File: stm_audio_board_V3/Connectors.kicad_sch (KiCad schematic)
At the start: 6 parts, among them J2 STlink_DISP_MCU, J2 STlink_DSP

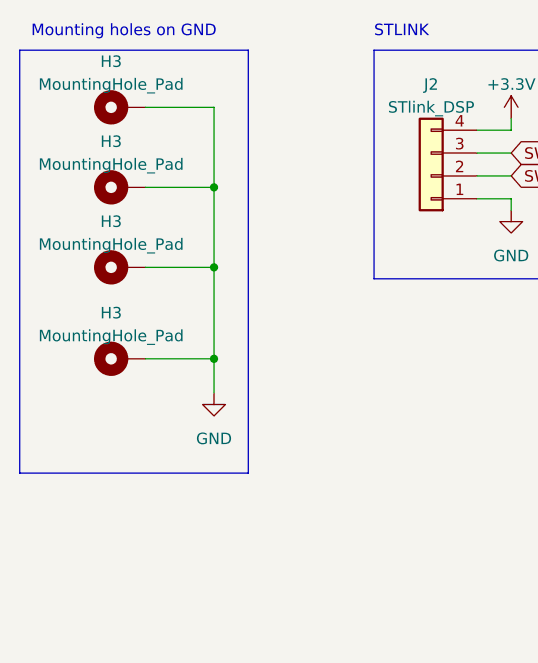
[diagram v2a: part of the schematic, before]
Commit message: PCB design is finished
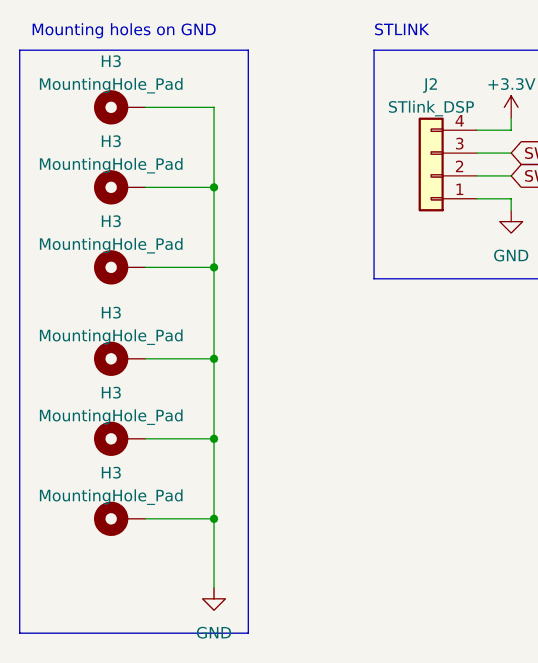
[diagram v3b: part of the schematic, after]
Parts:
- added H3 (x2): MountingHole_Pad, MountingHole:MountingHole_3.2mm_M3_DIN965_Pad, symbol Mechanical:MountingHole_Pad
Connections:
- net GND: now also H3.1, H3.1
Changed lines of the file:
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@@
   (junction (at 113.03 48.26) (diameter 0) (color 0 0 0 0)
   )
+  (junction (at 113.03 76.2) (diameter 0) (color 0 0 0 0)
+  )
+  (junction (at 113.03 67.31) (diameter 0) (color 0 0 0 0)
+  )
   (junction (at 113.03 39.37) (diameter 0) (color 0 0 0 0)
   )
-  (wire (pts (xy 113.03 62.23) (xy 113.03 58.42))
+  (wire (pts (xy 113.03 83.82) (xy 113.03 76.2))
     (stroke (width 0) (type default))
   )
@@
     (stroke (width 0) (type default))
   )
+  (wire (pts (xy 105.41 76.2) (xy 113.03 76.2))
+    (stroke (width 0) (type default))
+  )
+  (wire (pts (xy 113.03 76.2) (xy 113.03 67.31))
+    (stroke (width 0) (type default))
+  )
+  (wire (pts (xy 105.41 67.31) (xy 113.03 67.31))
+    (stroke (width 0) (type default))
+  )
   (wire (pts (xy 105.41 48.26) (xy 113.03 48.26))
     (stroke (width 0) (type default))
@@
     (stroke (width 0) (type default))
   )
+  (wire (pts (xy 113.03 67.31) (xy 113.03 58.42))
+    (stroke (width 0) (type default))
+  )
   (wire (pts (xy 142.24 33.02) (xy 146.05 33.02))
     (stroke (width 0) (type default))
@@
   )
   (text_box ""
-    (at 91.44 24.13 0) (size 25.4 46.99)
+    (at 91.44 24.13 0) (size 25.4 64.77)
     (stroke (width 0) (type default))
     (fill (type none))
@@
     )
   )
+  (symbol (lib_id "Mechanical:MountingHole_Pad") (at 102.87 67.31 90) (unit 1)
+    (in_bom yes) (on_board yes) (dnp no) (fields_autoplaced)
+    (property "Reference" "H3" (at 101.6 62.23 90)
+      (effects (font (size 1.27 1.27)))
+    )
+    (property "Value" "MountingHole_Pad" (at 101.6 64.77 90)
+      (effects (font (size 1.27 1.27)))
+    )
+    (property "Footprint" "MountingHole:MountingHole_3.2mm_M3_DIN965_Pad" (at 102.87 67.31 0)
+      (effects (font (size 1.27 1.27)) hide)
+    )
+    (property "Datasheet" "~" (at 102.87 67.31 0)
+      (effects (font (size 1.27 1.27)) hide)
+    )
+    (pin "1")
+    (instances
+      (project "stm_audio_board_V3"
+        (path "/6997cf63-2615-4e49-9471-e7da1b6bae71"
+          (reference "H3") (unit 1)
+        )
+        (path "/6997cf63-2615-4e49-9471-e7da1b6bae71/2eb2ee8f-ab98-4666-97f0-bfacb073bc88"
+          (reference "H4") (unit 1)
+        )
+        (path "/6997cf63-2615-4e49-9471-e7da1b6bae71/6424856c-1346-4018-a943-0d16008c9545"
+          (reference "H5") (unit 1)
+        )
+      )
+    )
+  )
   (symbol (lib_id "Mechanical:MountingHole_Pad") (at 102.87 58.42 90) (unit 1)
     (in_bom yes) (on_board yes) (dnp no) (fields_autoplaced)
@@
         (path "/6997cf63-2615-4e49-9471-e7da1b6bae71/6424856c-1346-4018-a943-0d16008c9545"
           (reference "#PWR034") (unit 1)
+        )
+      )
+    )
+  )
+  (symbol (lib_id "Mechanical:MountingHole_Pad") (at 102.87 76.2 90) (unit 1)
+    (in_bom yes) (on_board yes) (dnp no) (fields_autoplaced)
+    (property "Reference" "H3" (at 101.6 71.12 90)
+      (effects (font (size 1.27 1.27)))
+    )
+    (property "Value" "MountingHole_Pad" (at 101.6 73.66 90)
+      (effects (font (size 1.27 1.27)))
+    )
+    (property "Footprint" "MountingHole:MountingHole_3.2mm_M3_DIN965_Pad" (at 102.87 76.2 0)
+      (effects (font (size 1.27 1.27)) hide)
+    )
+    (property "Datasheet" "~" (at 102.87 76.2 0)
+      (effects (font (size 1.27 1.27)) hide)
+    )
+    (pin "1")
+    (instances
+      (project "stm_audio_board_V3"
+        (path "/6997cf63-2615-4e49-9471-e7da1b6bae71"
+          (reference "H3") (unit 1)
+        )
+        (path "/6997cf63-2615-4e49-9471-e7da1b6bae71/2eb2ee8f-ab98-4666-97f0-bfacb073bc88"
+          (reference "H4") (unit 1)
+        )
+        (path "/6997cf63-2615-4e49-9471-e7da1b6bae71/6424856c-1346-4018-a943-0d16008c9545"
+          (reference "H6") (unit 1)
         )
       )
@@
     )
   )
-  (symbol (lib_id "power:GND") (at 113.03 62.23 0) (unit 1)
-    (in_bom yes) (on_board yes) (dnp no) (fields_autoplaced)
-    (property "Reference" "#PWR02" (at 113.03 68.58 0)
-      (effects (font (size 1.27 1.27)) hide)
-    )
-    (property "Value" "GND" (at 113.03 67.31 0)
-      (effects (font (size 1.27 1.27)))
-    )
-    (property "Footprint" "" (at 113.03 62.23 0)
-      (effects (font (size 1.27 1.27)) hide)
-    )
-    (property "Datasheet" "" (at 113.03 62.23 0)
-      (effects (font (size 1.27 1.27)) hide)
-    )
+  (symbol (lib_id "power:GND") (at 113.03 83.82 0) (unit 1)
+    (in_bom yes) (on_board yes) (dnp no) (fields_autoplaced)
+    (property "Reference" "#PWR02" (at 113.03 90.17 0)
+      (effects (font (size 1.27 1.27)) hide)
+    )
+    (property "Value" "GND" (at 113.03 88.9 0)
+      (effects (font (size 1.27 1.27)))
+    )
+    (property "Footprint" "" (at 113.03 83.82 0)
+      (effects (font (size 1.27 1.27)) hide)
+    )
+    (property "Datasheet" "" (at 113.03 83.82 0)
+      (effects (font (size 1.27 1.27)) hide)
+    )
